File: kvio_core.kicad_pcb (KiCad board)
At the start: 6 copper layers, 60 x 41 mm, 214 parts, among them J1001 16-pin_FFC_(SFV16R), J1101 16-pin_FFC_(SFV16R), J1301 USB3_B_Micro, J301 Conn_01x06_Male, J401 16-pin_FFC_(SFV16R), J501 16-pin_FFC_(SFV16R), J601 16-pin_FFC_(SFV16R), J701 16-pin_FFC_(SFV16R), J801 16-pin_FFC_(SFV16R), J901 16-pin_FFC_(SFV16R), U1001 EMI8143, U101 xc7a100t-csg324, U1101 EMI8143, U1201 MT41J128M16JT-125:K, U1301 FT601Q, U1302 EMI8143, U201 FAN53541, U202 FAN53541, U203 FAN53541, U204 FAN53541, U301 MX25L3233F, U302 MAX809, U401 EMI8143, U501 EMI8143, U601 EMI8143, U701 EMI8143, U801 EMI8143, U901 EMI8143, Y1301 Crystal_GND24_Small

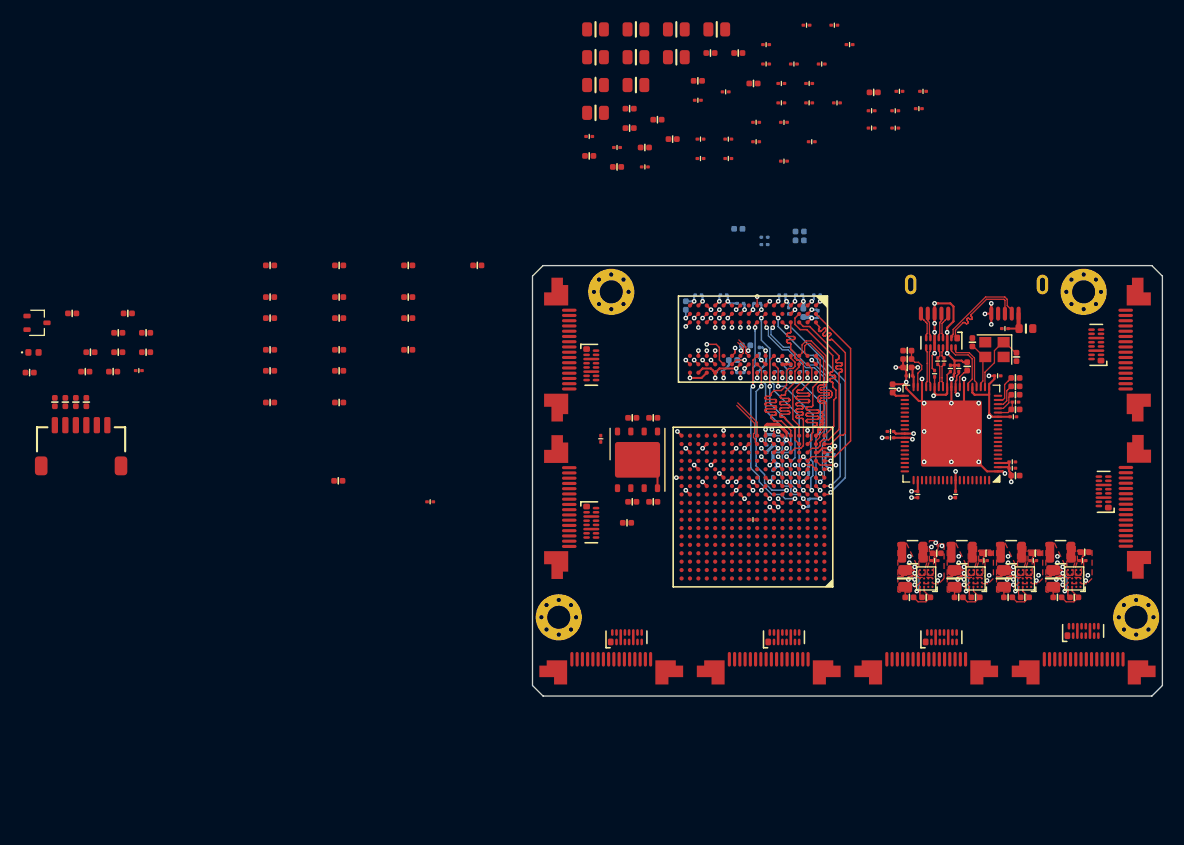
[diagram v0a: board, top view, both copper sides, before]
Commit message: More layout and design
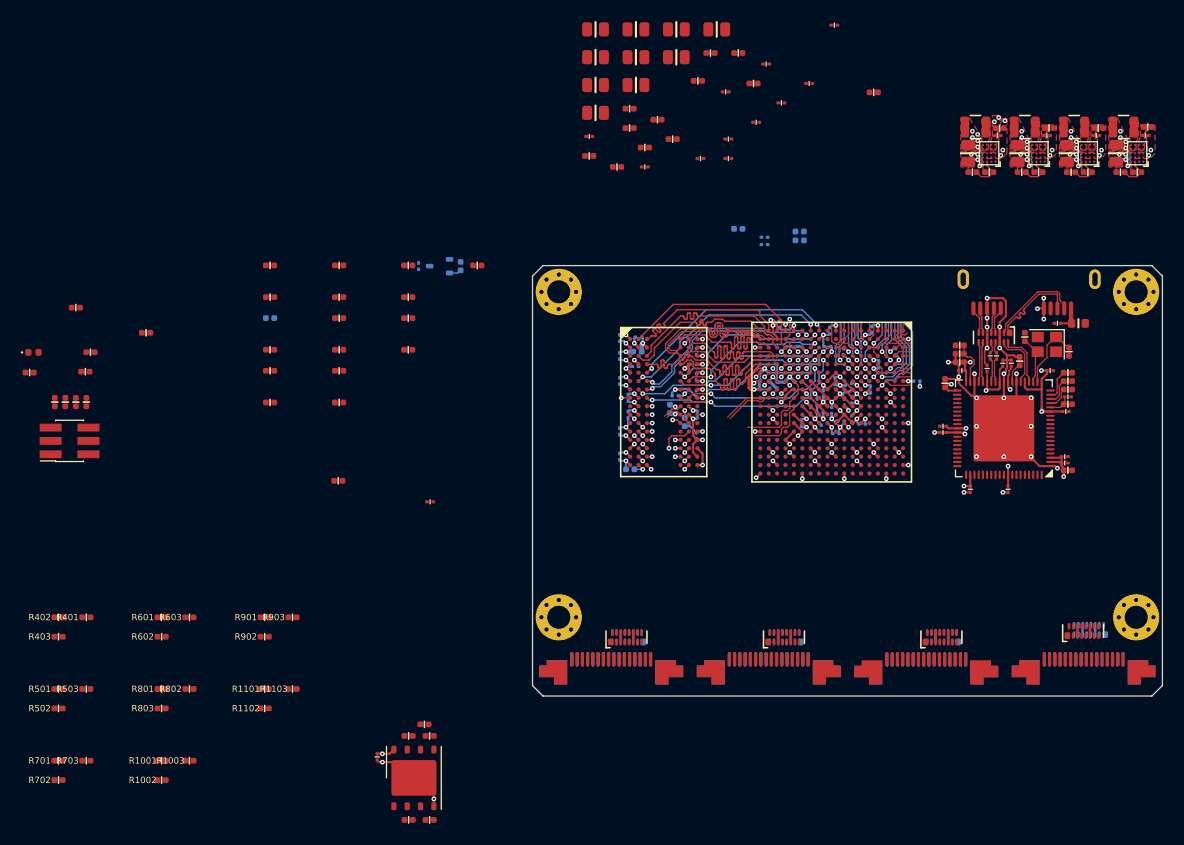
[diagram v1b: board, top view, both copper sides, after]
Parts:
- removed R304, R305, R306, R309: 1k, passive:R_0402
- added R1001: 100, passive:R_0402, F.Cu at (128.7, 136.2)
- added R1002: 100, passive:R_0402, F.Cu at (128.7, 138.0)
- added R1003: 100, passive:R_0402, F.Cu at (131.3, 136.2)
- added R1101: 100, passive:R_0402, F.Cu at (138.5, 129.3)
- added R1102: 100, passive:R_0402, F.Cu at (138.5, 131.2)
- added R1103: 100, passive:R_0402, F.Cu at (141.1, 129.3)
- added R401: 100, passive:R_0402, F.Cu at (121.5, 122.5)
- added R402: 100, passive:R_0402, F.Cu at (118.8, 122.5)
- added R403: 100, passive:R_0402, F.Cu at (118.8, 124.3)
- added R501: 100, passive:R_0402, F.Cu at (118.8, 129.3)
- added R502: 100, passive:R_0402, F.Cu at (118.8, 131.2)
- added R503: 100, passive:R_0402, F.Cu at (121.5, 129.3)
- added R601: 100, passive:R_0402, F.Cu at (128.7, 122.5)
- added R602: 100, passive:R_0402, F.Cu at (128.7, 124.3)
- added R603: 100, passive:R_0402, F.Cu at (131.3, 122.5)
- added R701: 100, passive:R_0402, F.Cu at (118.8, 136.2)
- added R702: 100, passive:R_0402, F.Cu at (118.8, 138.0)
- added R703: 100, passive:R_0402, F.Cu at (121.5, 136.2)
- added R801: 100, passive:R_0402, F.Cu at (128.7, 129.3)
- added R802: 100, passive:R_0402, F.Cu at (131.3, 129.3)
- added R803: 100, passive:R_0402, F.Cu at (128.7, 131.2)
- added R901: 100, passive:R_0402, F.Cu at (138.5, 122.5)
- added R902: 100, passive:R_0402, F.Cu at (138.5, 124.3)
- added R903: 100, passive:R_0402, F.Cu at (141.1, 122.5)
- C216, C221, C227, C231, C233, C237, C241, C245, C249, C253, C254, C255, C261, C262, C263, C264, C265, C266, C267, C268, C269, C270, C285, C302, FB201, J1001, J1101, J401, J501, R310, U1001, U1101, U302, U401, U501: moved to B.Cu
- J301: footprint connectors:jst-sh-hor-6 -> Connector_PinSocket_1.27mm:PinSocket_2x03_P1.27mm_Vertical_SMD
- R1204: value 80 -> 100
- R301, R311, R312, R313, R314, R317, R318, R319, R320: value 33 -> 100
- R307, R315, R316: value 10k -> 4.7k
- moved C271 40.9 mm to (222.6, 75.8)
- moved C272 40.9 mm to (222.4, 76.6)
- moved C273 40.9 mm to (219.6, 78.3)
- moved C274 40.9 mm to (213.2, 75.9)
- moved C275 40.9 mm to (213.0, 76.6)
- moved C276 40.9 mm to (210.2, 78.3)
- moved C277 40.9 mm to (208.5, 75.9)
- moved C278 40.9 mm to (208.3, 76.6)
- moved C279 40.9 mm to (205.5, 78.3)
- moved C280 40.9 mm to (217.9, 75.9)
- moved C281 40.9 mm to (217.7, 76.6)
- moved C282 40.9 mm to (214.9, 78.3)
- moved L201 40.9 mm to (220.3, 75.8)
- moved L202 40.9 mm to (210.9, 75.8)
- moved L203 40.9 mm to (206.2, 75.8)
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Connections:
- C1305 pad 1: /USB3 Interface/3V3 -> +3V3
- C1306 pad 1: /USB3 Interface/3V3 -> +3V3
- C1308 pad 1: /USB3 Interface/3V3 -> +3V3
- C1309 pad 1: /USB3 Interface/3V3 -> +3V3
- C1313 pad 1: /USB3 Interface/3V3 -> +3V3
- C1314 pad 1: /USB3 Interface/3V3 -> +3V3
- C1316 pad 1: /USB3 Interface/3V3 -> +3V3
- C1317 pad 1: /USB3 Interface/3V3 -> +3V3
- C301 pad 2: /Config/3V3 -> +3V3
- C302 pad 2: /Config/3V3 -> +3V3
- R1302 pad 1: /USB3 Interface/3V3 -> +3V3
- R1303 pad 1: /USB3 Interface/3V3 -> +3V3
- R302 pad 2: /Config/3V3 -> +3V3
- R307 pad 1: /Config/3V3 -> +3V3
- R308 pad 1: /Config/3V3 -> +3V3
- R315 pad 1: /Config/3V3 -> +3V3
- R316 pad 1: /Config/3V3 -> +3V3
- U101 pad P11: /Config/CFG_MODE2 -> GND
- U101 pad P12: /Config/CFG_MODE0 -> +3V3
- U101 pad P13: /Config/CFG_MODE1 -> GND
- U101 pad P8: /Config/3V3 -> +3V3
- U101 pad P9: /Config/CFG_PROGRAM_B -> /Config/CFG_INIT_B
- U1301 pad 14: /USB3 Interface/3V3 -> +3V3
- U1301 pad 20: /USB3 Interface/3V3 -> +3V3
- U1301 pad 24: /USB3 Interface/3V3 -> +3V3
- U1301 pad 28: /USB3 Interface/3V3 -> +3V3
- U1301 pad 38: /USB3 Interface/3V3 -> +3V3
- U1301 pad 49: /USB3 Interface/3V3 -> +3V3
- U1301 pad 59: /USB3 Interface/3V3 -> +3V3
- U1301 pad 68: /USB3 Interface/3V3 -> +3V3
- U301 pad 8: /Config/3V3 -> +3V3
- U302 pad 3: /Config/3V3 -> +3V3
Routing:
- net GND: track 98.2 -> 147.8 mm, vias 83 -> 105
- net +3V3: track 7.87 -> 42.8 mm, vias 11 -> 33
- net +1V0: track 7.31 -> 31.9 mm, vias 10 -> 15
- net /USB3 Interface/3V3: track 19.4 -> 0.00 mm, vias 7 -> 0
- net +1V8: track 4.48 -> 15.9 mm, vias 5 -> 10
- net /DDR Memory/A4: track 21.5 -> 12.0 mm
- net /USB3 Interface/DATA_21: track 0.00 -> 8.69 mm, vias 0 -> 1
- net /USB3 Interface/DATA_7: track 0.00 -> 8.58 mm, vias 0 -> 1
- net /Config/CFG_INIT_B: track 0.00 -> 8.55 mm
- net /USB3 Interface/DATA_12: track 0.00 -> 8.34 mm, vias 0 -> 1
- net /USB3 Interface/DATA_1: track 0.00 -> 6.05 mm, vias 0 -> 1
- net /Config/CFG_DONE: track 0.00 -> 5.97 mm
- net /USB3 Interface/TXE_N: track 0.00 -> 5.93 mm, vias 0 -> 1
- net /USB3 Interface/DATA_10: track 0.00 -> 5.19 mm, vias 0 -> 1
- net /USB3 Interface/DATA_0: track 0.00 -> 5.16 mm, vias 0 -> 1
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- added copper zone on GND_PWR2, net +1V0
- added copper zone on GND_PWR2, net +1V8
